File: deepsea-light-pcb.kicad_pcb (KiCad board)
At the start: 2 copper layers, 96.3 x 60.8 mm, 6 parts, among them CN1 XT60PW-M, U1 Pico, U2 2604-1106, U3 2604-1106, U4 2604-1106, U5 2604-1106

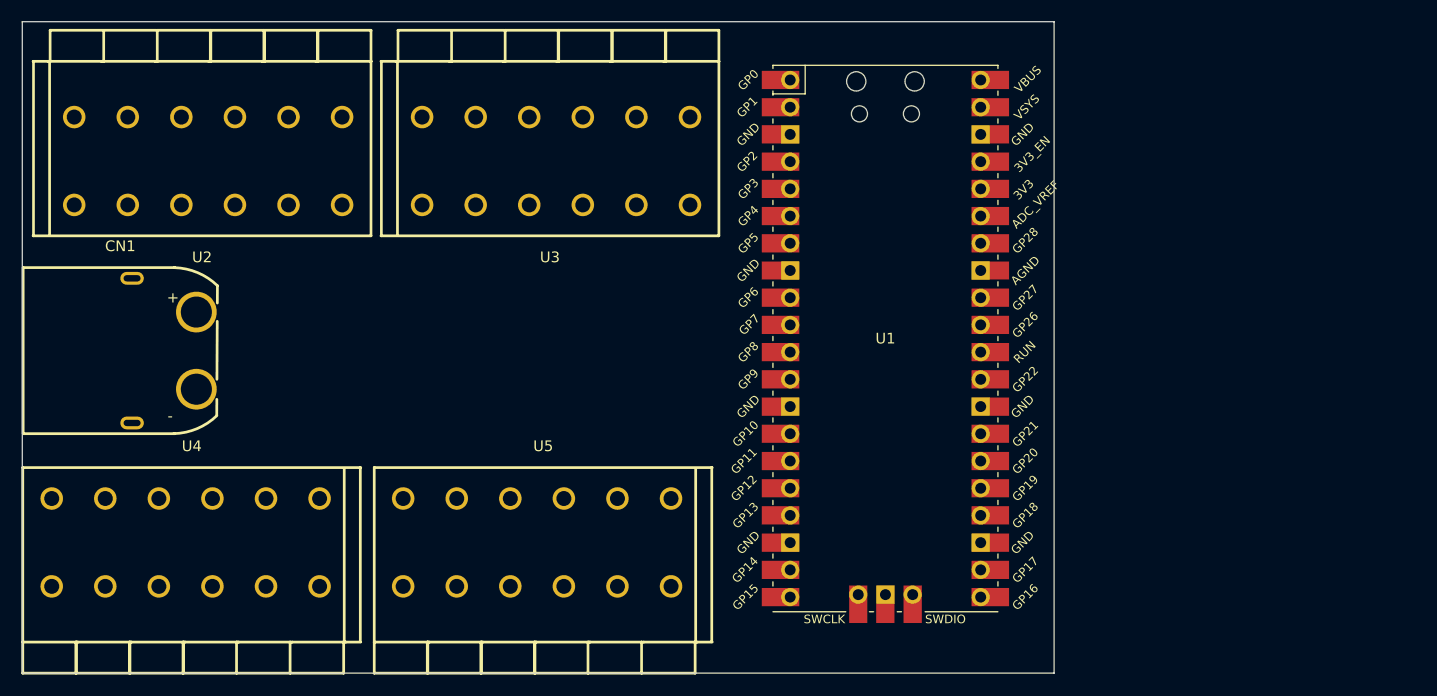
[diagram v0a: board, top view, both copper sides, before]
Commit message: Updates
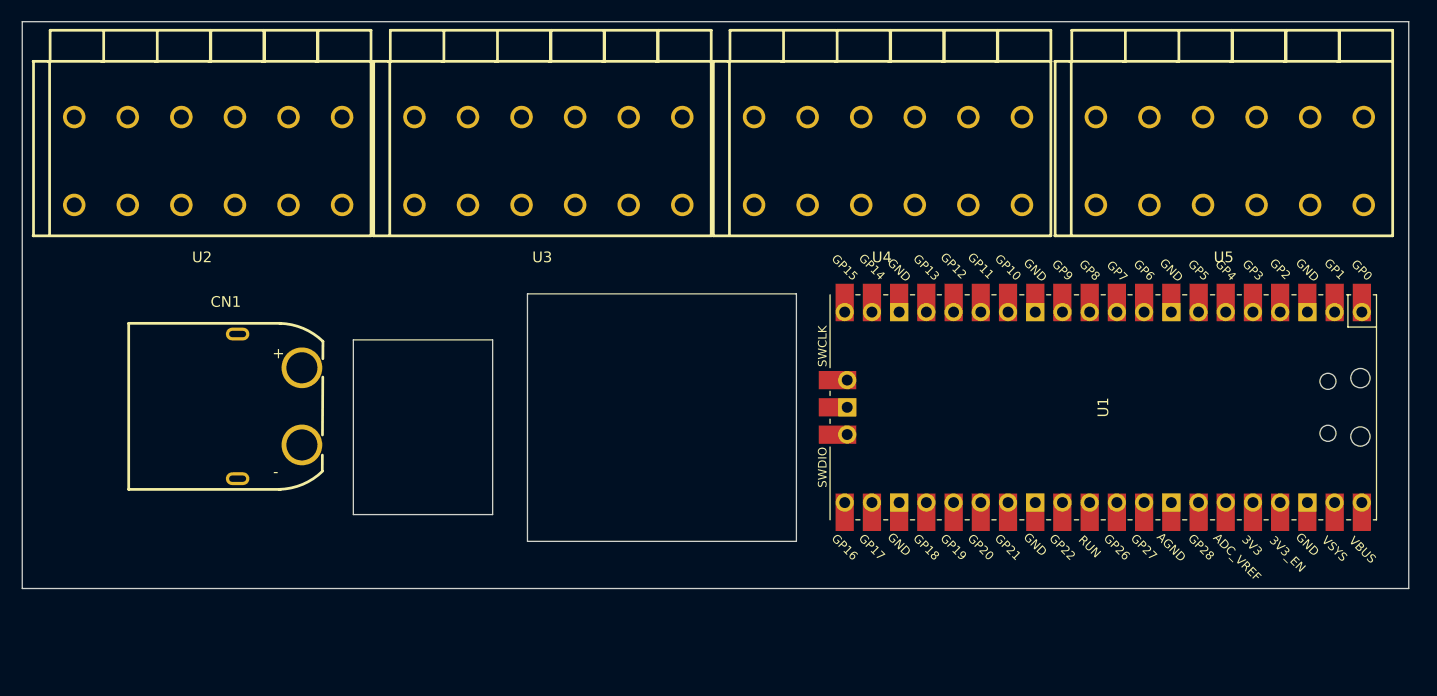
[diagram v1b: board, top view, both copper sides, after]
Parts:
- moved U4 74.6 mm to (176.8, 67.3), turned to 180 degrees
- moved U5 73.8 mm to (208.8, 67.3), turned to 180 degrees
- moved U1 21.3 mm to (196.9, 90.3), turned to -90 degrees
- moved CN1 11.1 mm to (119.2, 90.2)
- moved U3 0.72 mm to (145.2, 67.3)
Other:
- board size 96.3 x 60.8 mm -> 129.4 x 52.9 mm

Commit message: Updates
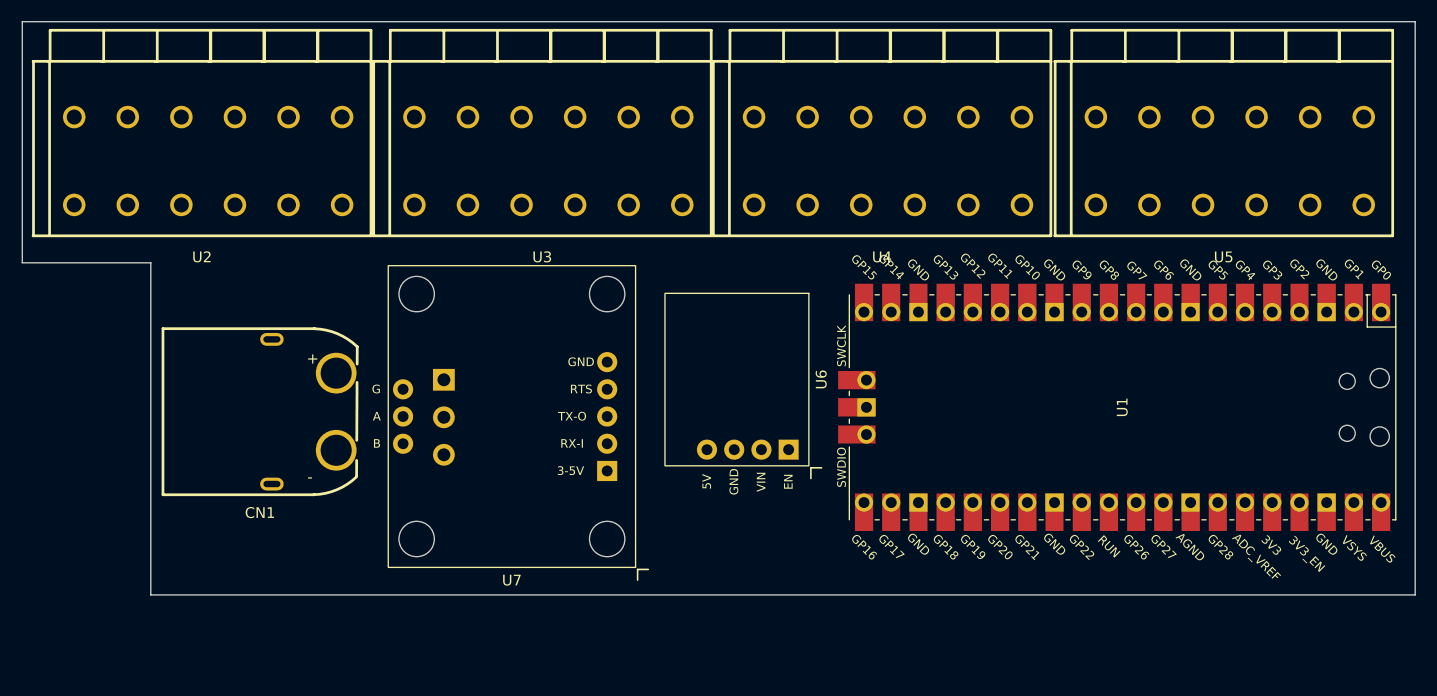
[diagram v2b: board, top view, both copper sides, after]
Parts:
- added U6: SparkFun_BabyBuck_5V, Deepsea_light_lib:SparkFun_BabyBuck_5V, F.Cu at (162.8, 87.7)
- added U7: SparkFun_RS485_Breakout, Deepsea_light_lib:SparkFun_RS485_Breakout, F.Cu at (141.8, 91.2)
- moved CN1 3.24 mm to (122.4, 90.7)
- moved U1 1.80 mm to (198.7, 90.3)
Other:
- board size 129.4 x 52.9 mm -> 130 x 53.5 mm

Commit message: Update
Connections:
- U1 pad 13: unconnected-(U1-GND-Pad13) -> GND
- U1 pad 18: unconnected-(U1-GND-Pad18) -> GND
- U1 pad 23: unconnected-(U1-GND-Pad23) -> GND
- U1 pad 28: unconnected-(U1-GND-Pad28) -> GND
- U1 pad 3: unconnected-(U1-GND-Pad3) -> GND
- U1 pad 38: unconnected-(U1-GND-Pad38) -> GND
- U1 pad 40: unconnected-(U1-VBUS-Pad40) -> +5V
- U1 pad 8: unconnected-(U1-GND-Pad8) -> GND
- U6 pad 2: unconnected-(U6-VIN-Pad2) -> +24V
- U6 pad 3: unconnected-(U6-GND-Pad3) -> GND
- U6 pad 4: unconnected-(U6-VOUT-Pad4) -> +5V
- U7 pad 5: unconnected-(U7-GND-Pad5) -> GND
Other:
- copper layers 2 -> 4
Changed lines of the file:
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@@
 	(layers
 		(0 "F.Cu" signal)
+		(4 "In1.Cu" signal)
+		(6 "In2.Cu" signal)
 		(2 "B.Cu" signal)
 		(9 "F.Adhes" user "F.Adhesive")
@@
 			)
 			(layer "dielectric 1"
+				(type "prepreg")
+				(thickness 0.1)
+				(material "FR4")
+				(epsilon_r 4.5)
+				(loss_tangent 0.02)
+			)
+			(layer "In1.Cu"
+				(type "copper")
+				(thickness 0.035)
+			)
+			(layer "dielectric 2"
 				(type "core")
-				(thickness 1.51)
+				(thickness 1.24)
+				(material "FR4")
+				(epsilon_r 4.5)
+				(loss_tangent 0.02)
+			)
+			(layer "In2.Cu"
+				(type "copper")
+				(thickness 0.035)
+			)
+			(layer "dielectric 3"
+				(type "prepreg")
+				(thickness 0.1)
 				(material "FR4")
 				(epsilon_r 4.5)
@@
 		(capping no)
 		(filling no)
+		(zone_defaults)
 		(aux_axis_origin 96.05 54.3)
 		(grid_origin 96.05 54.3)
@@
 		(sheetname "/")
 		(sheetfile "deepsea-light-pcb.kicad_sch")
+		(units
+			(unit
+				(name "A")
+				(pins "1" "2" "3" "4" "5" "6")
+			)
+		)
 		(attr through_hole)
 		(duplicate_pad_numbers_are_jumpers no)
@@
 		(sheetname "/")
 		(sheetfile "deepsea-light-pcb.kicad_sch")
+		(units
+			(unit
+				(name "A")
+				(pins "2" "1" "3" "4")
+			)
+		)
 		(attr through_hole)
 		(duplicate_pad_numbers_are_jumpers no)
@@
 			(layers "*.Cu" "*.Mask")
 			(remove_unused_layers no)
-			(net "unconnected-(U6-VIN-Pad2)")
+			(net "+24V")
 			(pinfunction "VIN_2")
 			(pintype "power_in")
@@
 			(layers "*.Cu" "*.Mask")
 			(remove_unused_layers no)
-			(net "unconnected-(U6-GND-Pad3)")
+			(net "GND")
 			(pinfunction "GND_3")
 			(pintype "power_in")
@@
 			(layers "*.Cu" "*.Mask")
 			(remove_unused_layers no)
-			(net "unconnected-(U6-VOUT-Pad4)")
+			(net "+5V")
 			(pinfunction "VOUT_4")
 			(pintype "power_out")
@@
 		(sheetname "/")
 		(sheetfile "deepsea-light-pcb.kicad_sch")
+		(units
+			(unit
+				(name "A")
+				(pins "1" "2" "3" "4" "5" "6" "7" "8" "9" "10" "11" "12" "13" "14" "15"
+					"16" "17" "18" "19" "20" "41" "42" "43" "40" "39" "38" "37" "36" "35"
+					"34" "33" "32" "31" "30" "29" "28" "27" "26" "25" "24" "23" "22" "21"
+				)
+			)
+		)
 		(attr through_hole)
 		(duplicate_pad_numbers_are_jumpers no)
@@
 			(layers "*.Cu" "*.Mask")
 			(remove_unused_layers no)
-			(net "unconnected-(U1-GND-Pad3)")
+			(net "GND")
 			(pinfunction "GND_3")
 			(pintype "power_in")
@@
 			)
 			(layers "F.Cu" "F.Mask")
-			(net "unconnected-(U1-GND-Pad3)")
+			(net "GND")
 			(pinfunction "GND_3")
 			(pintype "power_in")
@@
 			(layers "*.Cu" "*.Mask")
 			(remove_unused_layers no)
-			(net "unconnected-(U1-GND-Pad8)")
+			(net "GND")
 			(pinfunction "GND_8")
 			(pintype "power_in")
@@
 			)
 			(layers "F.Cu" "F.Mask")
-			(net "unconnected-(U1-GND-Pad8)")
+			(net "GND")
 			(pinfunction "GND_8")
 			(pintype "power_in")
@@
 			(layers "*.Cu" "*.Mask")
 			(remove_unused_layers no)
-			(net "unconnected-(U1-GND-Pad13)")
+			(net "GND")
 			(pinfunction "GND_13")
 			(pintype "power_in")
@@
 			)
 			(layers "F.Cu" "F.Mask")
-			(net "unconnected-(U1-GND-Pad13)")
+			(net "GND")
 			(pinfunction "GND_13")
 			(pintype "power_in")
@@
 			(layers "*.Cu" "*.Mask")
 			(remove_unused_layers no)
-			(net "unconnected-(U1-GND-Pad18)")
+			(net "GND")
 			(pinfunction "GND_18")
 			(pintype "power_in")
@@
 			)
 			(layers "F.Cu" "F.Mask")
-			(net "unconnected-(U1-GND-Pad18)")
+			(net "GND")
 			(pinfunction "GND_18")
 			(pintype "power_in")
@@
 			(layers "*.Cu" "*.Mask")
 			(remove_unused_layers no)
-			(net "unconnected-(U1-GND-Pad23)")
+			(net "GND")
 			(pinfunction "GND_23")
 			(pintype "power_in")
@@
 			)
 			(layers "F.Cu" "F.Mask")
-			(net "unconnected-(U1-GND-Pad23)")
+			(net "GND")
 			(pinfunction "GND_23")
 			(pintype "power_in")
@@
 			(layers "*.Cu" "*.Mask")
 			(remove_unused_layers no)
-			(net "unconnected-(U1-GND-Pad28)")
+			(net "GND")
 			(pinfunction "GND_28")
 			(pintype "power_in")
@@
 			)
 			(layers "F.Cu" "F.Mask")
-			(net "unconnected-(U1-GND-Pad28)")
+			(net "GND")
 			(pinfunction "GND_28")
 			(pintype "power_in")
@@
 			(layers "*.Cu" "*.Mask")
 			(remove_unused_layers no)
-			(net "unconnected-(U1-GND-Pad38)")
+			(net "GND")
 			(pinfunction "GND_38")
 			(pintype "bidirectional")
@@
 			)
 			(layers "F.Cu" "F.Mask")
-			(net "unconnected-(U1-GND-Pad38)")
+			(net "GND")
 			(pinfunction "GND_38")
 			(pintype "bidirectional")
@@
 			(layers "*.Cu" "*.Mask")
 			(remove_unused_layers no)
-			(net "unconnected-(U1-VBUS-Pad40)")
+			(net "+5V")
 			(pinfunction "VBUS_40")
 			(pintype "power_in")
@@
 			)
 			(layers "F.Cu" "F.Mask")
-			(net "unconnected-(U1-VBUS-Pad40)")
+			(net "+5V")
 			(pinfunction "VBUS_40")
 			(pintype "power_in")
@@
 		(sheetname "/")
 		(sheetfile "deepsea-light-pcb.kicad_sch")
+		(units
+			(unit
+				(name "A")
+				(pins "1" "2" "3" "4" "5" "7" "8" "6")
+			)
+		)
 		(attr through_hole)
 		(duplicate_pad_numbers_are_jumpers no)
@@
 			(layers "*.Cu" "*.Mask")
 			(remove_unused_layers no)
-			(net "unconnected-(U7-GND-Pad5)")
+			(net "GND")
 			(pinfunction "GND_5")
 			(pintype "power_in")
@@
 		(sheetname "/")
 		(sheetfile "deepsea-light-pcb.kicad_sch")
+		(units
+			(unit
+				(name "A")
+				(pins "1" "2" "3" "4" "5" "6")
+			)
+		)
 		(attr through_hole)
 		(duplicate_pad_numbers_are_jumpers no)
@@
 		(sheetname "/")
 		(sheetfile "deepsea-light-pcb.kicad_sch")
+		(units
+			(unit
+				(name "A")
+				(pins "1" "2" "3" "4" "5" "6")
+			)
+		)
 		(attr through_hole)
 		(duplicate_pad_numbers_are_jumpers no)
@@
 		(sheetname "/")
 		(sheetfile "deepsea-light-pcb.kicad_sch")
+		(units
+			(unit
+				(name "A")
+				(pins "1" "2" "3" "4" "5" "6")
+			)
+		)
 		(attr through_hole)
 		(duplicate_pad_numbers_are_jumpers no)
@@
 		(sheetname "/")
 		(sheetfile "deepsea-light-pcb.kicad_sch")
+		(units
+			(unit
+				(name "A")
+				(pins "1" "2" "4" "3")
+			)
+		)
 		(attr through_hole)
 		(duplicate_pad_numbers_are_jumpers no)

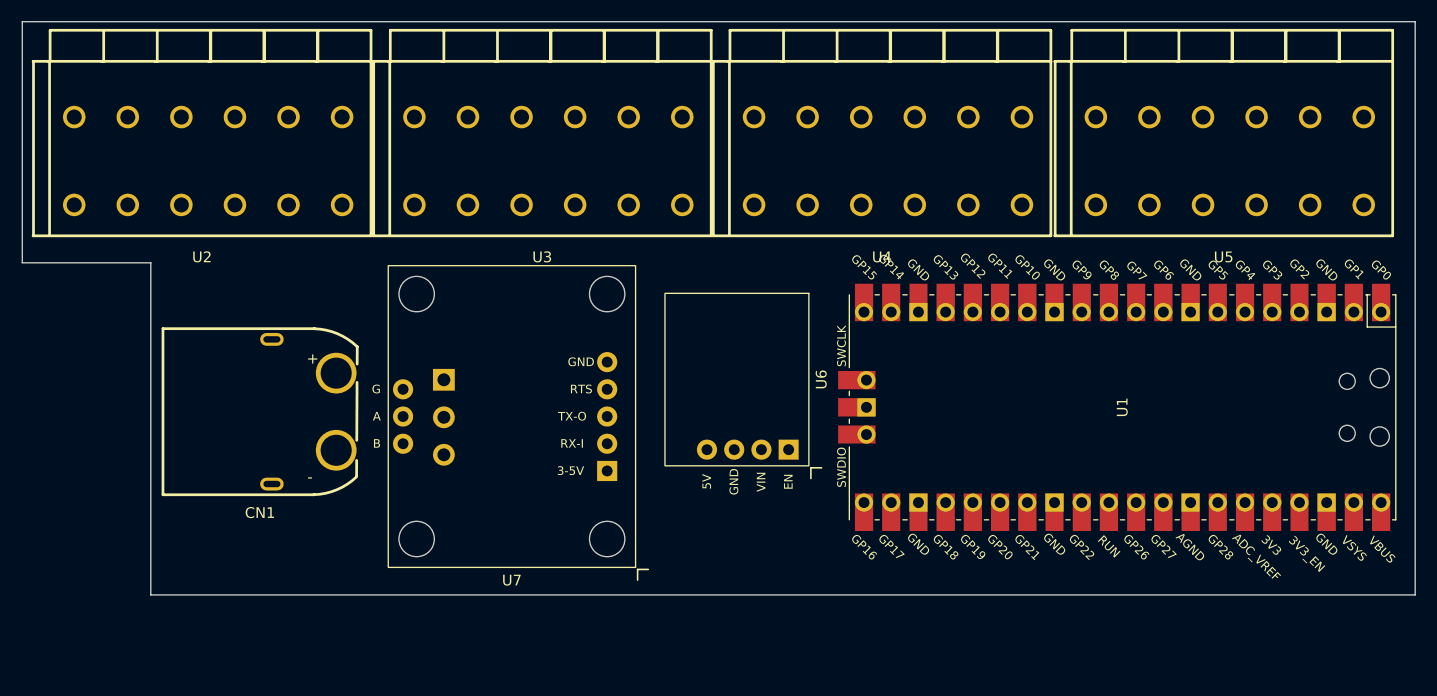
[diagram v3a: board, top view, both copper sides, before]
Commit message: updates
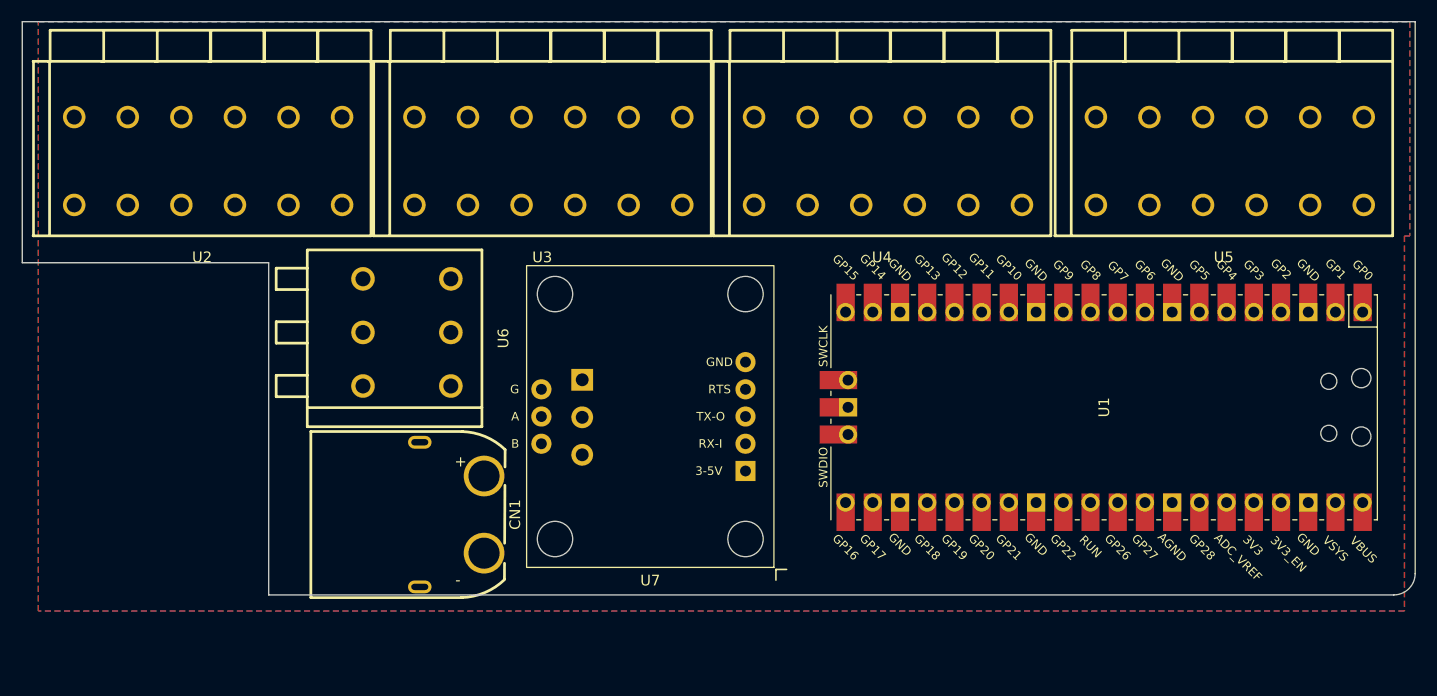
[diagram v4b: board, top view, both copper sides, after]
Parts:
- U6: value SparkFun_BabyBuck_5V -> 2604-1103; footprint Deepsea_light_lib:SparkFun_BabyBuck_5V -> Deepsea_light_lib:CONN-TH_2604-1103
- moved U6 31.1 mm to (132.0, 83.3)
- moved CN1 16.8 mm to (136.2, 100.3)
- moved U7 12.9 mm to (154.7, 91.2)
- moved U1 1.72 mm to (197.0, 90.3)
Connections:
- CN1 pad 1: GND -> LIGHT_GND
- CN1 pad 3: unconnected-(CN1-Pad3) -> LIGHT_GND
- CN1 pad 4: unconnected-(CN1-Pad4) -> LIGHT_GND
- U1 pad 1: unconnected-(U1-GPIO0-Pad1) -> /LIGHTS_TX
- U1 pad 2: unconnected-(U1-GPIO1-Pad2) -> /LIGHTS_RX
- U1 pad 21: unconnected-(U1-GPIO16-Pad21) -> /PWM_INPUT
- U1 pad 25: unconnected-(U1-GPIO19-Pad25) -> /LIGHTS_RTS
- U1 pad 39: unconnected-(U1-VSYS-Pad39) -> +5V
- U1 pad 40: +5V -> unconnected-(U1-VBUS-Pad40)
- U2 pad 2: GND -> LIGHT_GND
- U3 pad 2: GND -> LIGHT_GND
- U4 pad 2: GND -> LIGHT_GND
- U5 pad 2: GND -> LIGHT_GND
- U6 pad 1: unconnected-(U6-EN-Pad1) -> +5V
- U6 pad 2: +24V -> /PWM_INPUT
- U7 pad 1: unconnected-(U7-3-5V-Pad1) -> +5V
- U7 pad 2: unconnected-(U7-RX-I-Pad2) -> /LIGHTS_RX
- U7 pad 3: unconnected-(U7-TX-O-Pad3) -> /LIGHTS_TX
- U7 pad 4: unconnected-(U7-RTS-Pad4) -> /LIGHTS_RTS
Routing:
- added copper zone on In2.Cu, net +24V
- added copper zone on B.Cu, net LIGHT_GND
- added copper zone on F.Cu, net LIGHT_GND
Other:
- outline, holes or cut-outs redrawn
